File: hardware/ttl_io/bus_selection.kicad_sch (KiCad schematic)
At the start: 24 parts, among them SW2 SW_SPDT, U15 SN74LVC1G14DRL

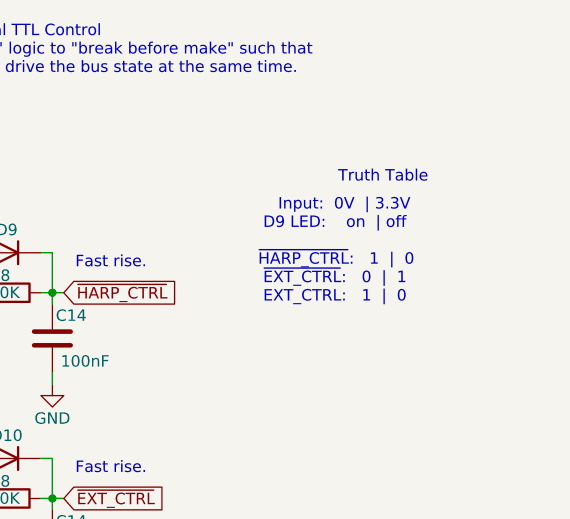
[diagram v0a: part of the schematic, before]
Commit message: update pcb
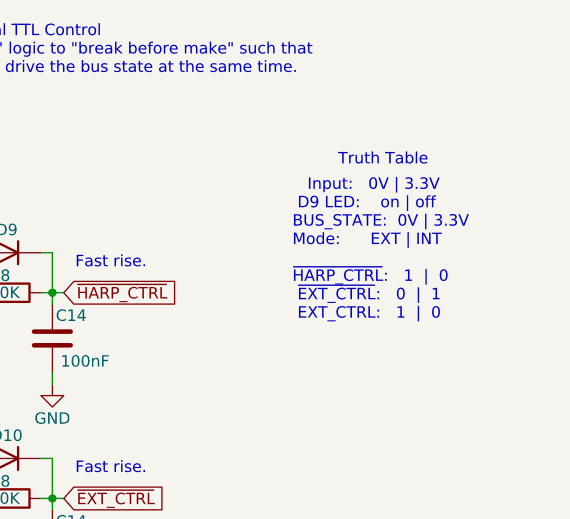
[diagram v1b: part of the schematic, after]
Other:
- note added: "Input: 0V | 3.3V D9 LED: on | off BUS_STATE: 0V | 3.3V Mode: EXT | INT ~{HARP_CTRL}: 1 | 0 ~{EXT_CTRL}: 0 | 1 EXT_CTRL: 1 | 0"
- note removed: "Input: 0V | 3.3V D9 LED: on | off ~{HARP_CTRL}: 1 | 0 ~{EXT_CTRL}: 0 | 1 EXT_CTRL: 1 | 0"
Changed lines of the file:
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@@
     (stroke (width 0) (type default))
   )
-  (text "Truth Table" (at 224.155 66.04 0)
+  (text "Truth Table" (at 224.155 64.135 0)
     (effects (font (size 1.27 1.27)) (justify left bottom))
   )
@@
     (effects (font (size 1.27 1.27)) (justify left bottom))
   )
-  (text "    Input:  0V  | 3.3V\n D9 LED:    on  | off\n\n~{HARP_CTRL}:   1  |  0\n ~{EXT_CTRL}:   0  |  1\n EXT_CTRL:   1  |  0"
-    (at 215.265 79.375 0)
+  (text "   Input:   0V | 3.3V\n D9 LED:    on | off\nBUS_STATE:  0V | 3.3V\nMode:      EXT | INT\n\n~{HARP_CTRL}:   1  |  0\n ~{EXT_CTRL}:   0  |  1\n EXT_CTRL:   1  |  0"
+    (at 219.075 81.28 0)
     (effects (font (face "Ubuntu Mono") (size 1.27 1.27)) (justify left bottom))
   )

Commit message: update pcb and bom
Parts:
- SW2: Notes 6V max -> 6V max, may not be washable.
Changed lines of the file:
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@@
       (effects (font (size 1.27 1.27)) hide)
     )
-    (property "Notes" "6V max" (at 113.665 107.315 90)
+    (property "Notes" "6V max, may not be washable." (at 113.665 107.315 90)
       (effects (font (size 1.27 1.27)) hide)
     )
